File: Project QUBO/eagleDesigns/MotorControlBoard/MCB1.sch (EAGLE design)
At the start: 33 parts, among them U1 PCA9685

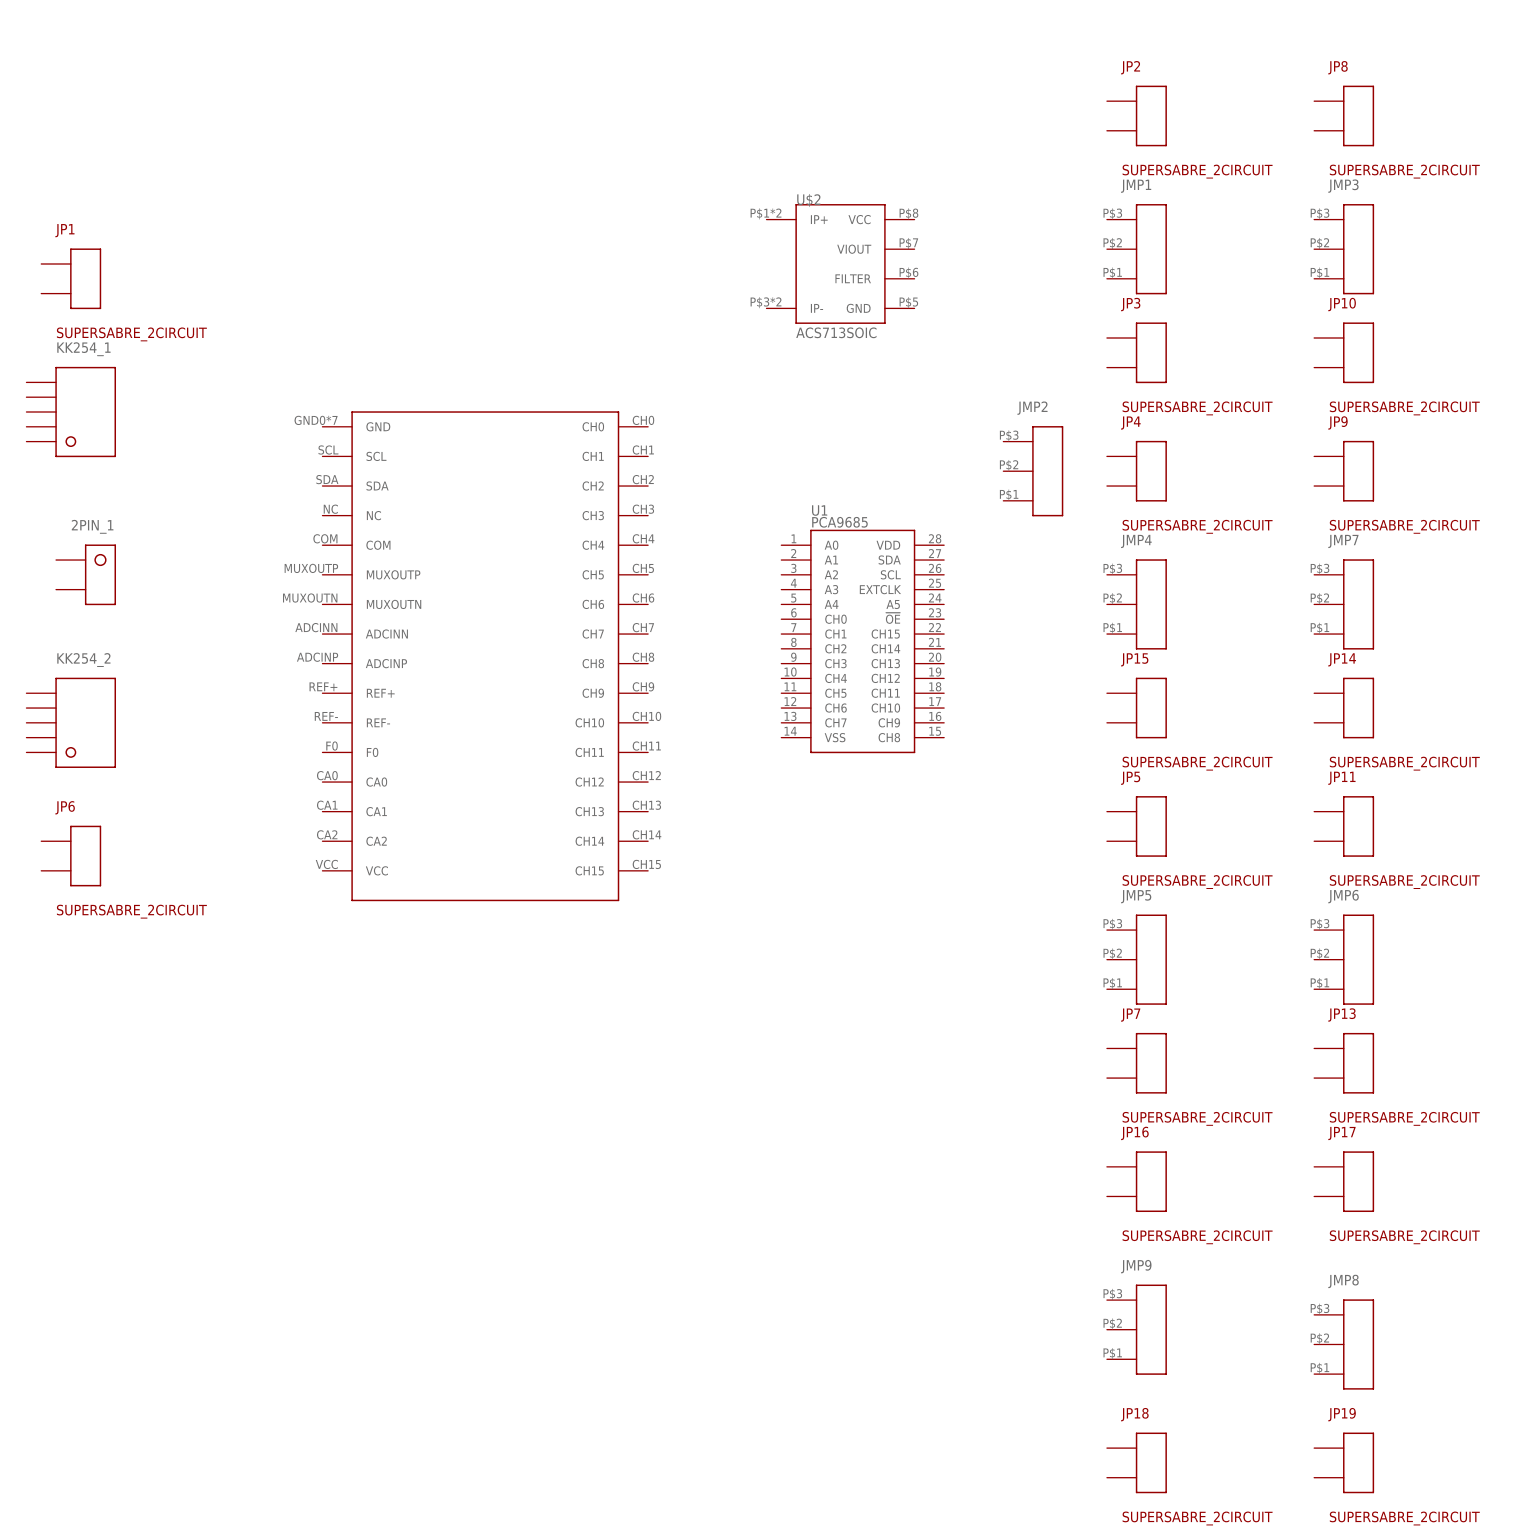
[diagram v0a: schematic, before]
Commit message: edited motor board
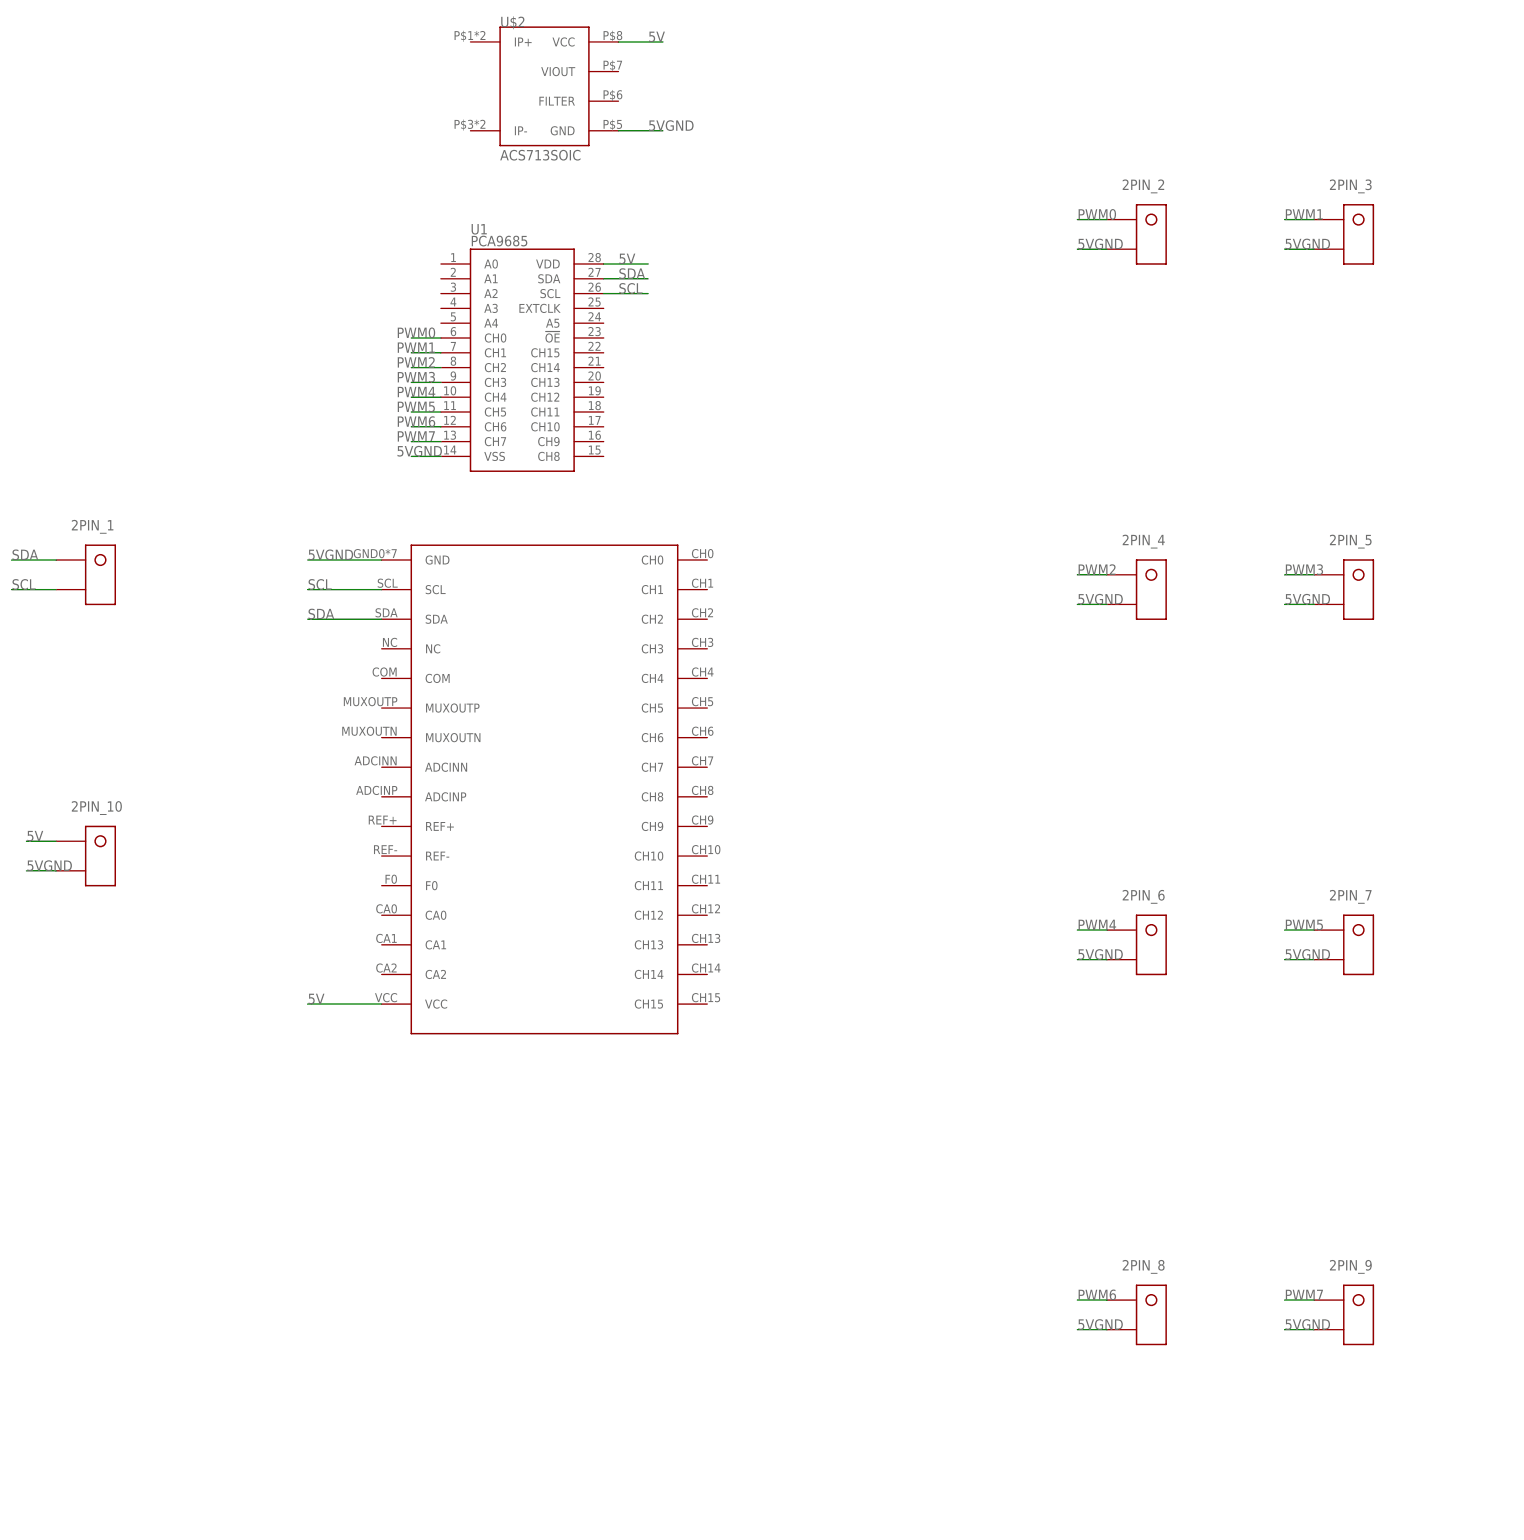
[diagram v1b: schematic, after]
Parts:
- removed JMP1, JMP2, JMP3, JMP4, JMP5, JMP6, JMP7, JMP8, JMP9: (no value), molex:KK254_VERT_3PIN22-10-2031
- removed JP1, JP10, JP11, JP13, JP14, JP15, JP16, JP17, JP18, JP19, JP2, JP3, JP4, JP5, JP6, JP7, JP8, JP9: SUPERSABRE_2CIRCUIT, molex:SUPERSABRE_2CIRCUIT
- removed KK254_1, KK254_2: (no value), molex:KK254_VERT_5PIN
- added 2PIN_10, 2PIN_2, 2PIN_3, 2PIN_4, 2PIN_5, 2PIN_6, 2PIN_7, 2PIN_8, 2PIN_9: (no value), molex:KK254_VERT_2PIN22-29-2021
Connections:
- new net 5V: 2PIN_10.P$1, U$1.VCC, U$2.VCC, U1.VDD
- new net 5VGND: 2PIN_10.P$2, 2PIN_2.P$2, 2PIN_3.P$2, 2PIN_4.P$2, 2PIN_5.P$2, 2PIN_6.P$2, 2PIN_7.P$2, 2PIN_8.P$2, 2PIN_9.P$2, U$1.GND, U$2.GND, U1.VSS
- new net PWM0: 2PIN_2.P$1, U1.CH0
- new net PWM1: 2PIN_3.P$1, U1.CH1
- new net PWM2: 2PIN_4.P$1, U1.CH2
- new net PWM3: 2PIN_5.P$1, U1.CH3
- new net PWM4: 2PIN_6.P$1, U1.CH4
- new net PWM5: 2PIN_7.P$1, U1.CH5
- new net PWM6: 2PIN_8.P$1, U1.CH6
- new net PWM7: 2PIN_9.P$1, U1.CH7
- new net SCL: 2PIN_1.P$2, U$1.SCL, U1.SCL
- new net SDA: 2PIN_1.P$1, U$1.SDA, U1.SDA
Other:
- moved on the sheet: U$2, U1
